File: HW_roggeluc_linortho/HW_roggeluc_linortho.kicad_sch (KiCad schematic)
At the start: 6 parts, among them P3 DIN41612_02x32_AB, P4 DIN41612_02x32_AB

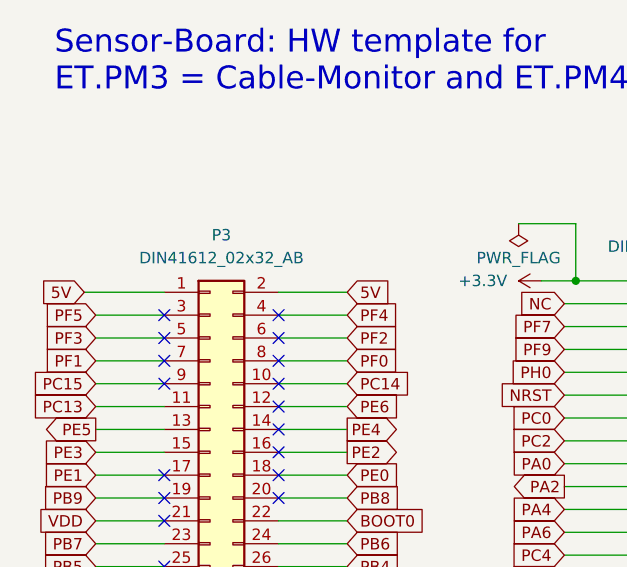
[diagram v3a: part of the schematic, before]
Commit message: PCB ORDERED
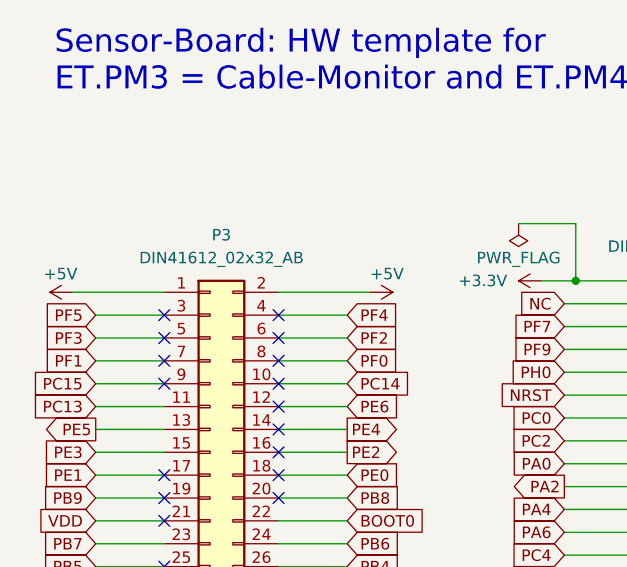
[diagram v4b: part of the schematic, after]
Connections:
- net 5V renamed +5V
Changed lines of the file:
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@@
 	(wire
 		(pts
-			(xy 50.8 41.91) (xy 58.42 41.91)
+			(xy 50.8 41.91) (xy 60.96 41.91)
 		)
 		(stroke
@@
 	(wire
 		(pts
-			(xy 29.21 41.91) (xy 38.1 41.91)
+			(xy 27.94 41.91) (xy 38.1 41.91)
 		)
 		(stroke
@@
 		)
 	)
-	(global_label "5V"
-		(shape input)
-		(at 29.21 41.91 180)
-		(fields_autoplaced yes)
-		(effects
-			(font
-				(size 1.27 1.27)
-			)
-			(justify right)
-		)
-		(property "Intersheetrefs" "${INTERSHEET_REFS}"
-			(at 23.9267 41.91 0)
-			(effects
-				(font
-					(size 1.27 1.27)
-				)
-				(justify right)
-				(hide yes)
-			)
-		)
-	)
 	(global_label "PD10"
 		(shape input)
@@
 		)
 	)
-	(global_label "5V"
-		(shape input)
-		(at 58.42 41.91 0)
-		(fields_autoplaced yes)
-		(effects
-			(font
-				(size 1.27 1.27)
-			)
-			(justify left)
-		)
-		(property "Intersheetrefs" "${INTERSHEET_REFS}"
-			(at 63.7033 41.91 0)
-			(effects
-				(font
-					(size 1.27 1.27)
-				)
-				(justify left)
-				(hide yes)
-			)
-		)
-	)
 	(global_label "PE4"
 		(shape output)
@@
 	)
 	(symbol
+		(lib_id "power:+5V")
+		(at 27.94 41.91 90)
+		(unit 1)
+		(exclude_from_sim no)
+		(in_bom yes)
+		(on_board yes)
+		(dnp no)
+		(property "Reference" "#PWR029"
+			(at 31.75 41.91 0)
+			(effects
+				(font
+					(size 1.27 1.27)
+				)
+				(hide yes)
+			)
+		)
+		(property "Value" "+5V"
+			(at 28.448 39.878 90)
+			(effects
+				(font
+					(size 1.27 1.27)
+				)
+				(justify left)
+			)
+		)
+		(property "Footprint" ""
+			(at 27.94 41.91 0)
+			(effects
+				(font
+					(size 1.27 1.27)
+				)
+				(hide yes)
+			)
+		)
+		(property "Datasheet" ""
+			(at 27.94 41.91 0)
+			(effects
+				(font
+					(size 1.27 1.27)
+				)
+				(hide yes)
+			)
+		)
+		(property "Description" "Power symbol creates a global label with name \"+5V\""
+			(at 27.94 41.91 0)
+			(effects
+				(font
+					(size 1.27 1.27)
+				)
+				(hide yes)
+			)
+		)
+		(pin "1"
+		)
+		(instances
+			(project "HW_roggeluc_linortho"
+				(path "/1f276d59-ad9b-4e70-a842-f3b7e562eb9b"
+					(reference "#PWR029")
+					(unit 1)
+				)
+			)
+		)
+	)
+	(symbol
 		(lib_id "power:GND")
 		(at 116.84 137.16 0)
@@
 					(unit 1)
 				)
+			)
+		)
+	)
+	(symbol
+		(lib_id "power:+5V")
+		(at 60.96 41.91 270)
+		(unit 1)
+		(exclude_from_sim no)
+		(in_bom yes)
+		(on_board yes)
+		(dnp no)
+		(property "Reference" "#PWR020"
+			(at 57.15 41.91 0)
+			(effects
+				(font
+					(size 1.27 1.27)
+				)
+				(hide yes)
+			)
+		)
+		(property "Value" "+5V"
+			(at 60.96 39.878 90)
+			(effects
+				(font
+					(size 1.27 1.27)
+				)
+				(justify left)
+			)
+		)
+		(property "Footprint" ""
+			(at 60.96 41.91 0)
+			(effects
+				(font
+					(size 1.27 1.27)
+				)
+				(hide yes)
+			)
+		)
+		(property "Datasheet" ""
+			(at 60.96 41.91 0)
+			(effects
+				(font
+					(size 1.27 1.27)
+				)
+				(hide yes)
+			)
+		)
+		(property "Description" "Power symbol creates a global label with name \"+5V\""
+			(at 60.96 41.91 0)
+			(effects
+				(font
+					(size 1.27 1.27)
+				)
+				(hide yes)
+			)
+		)
+		(pin "1"
+		)
+		(instances
+			(project "HW_roggeluc_linortho"
+				(path "/1f276d59-ad9b-4e70-a842-f3b7e562eb9b"
+					(reference "#PWR020")
+					(unit 1)
+				)
